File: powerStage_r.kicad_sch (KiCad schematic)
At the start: 19 parts, among them J3 motor

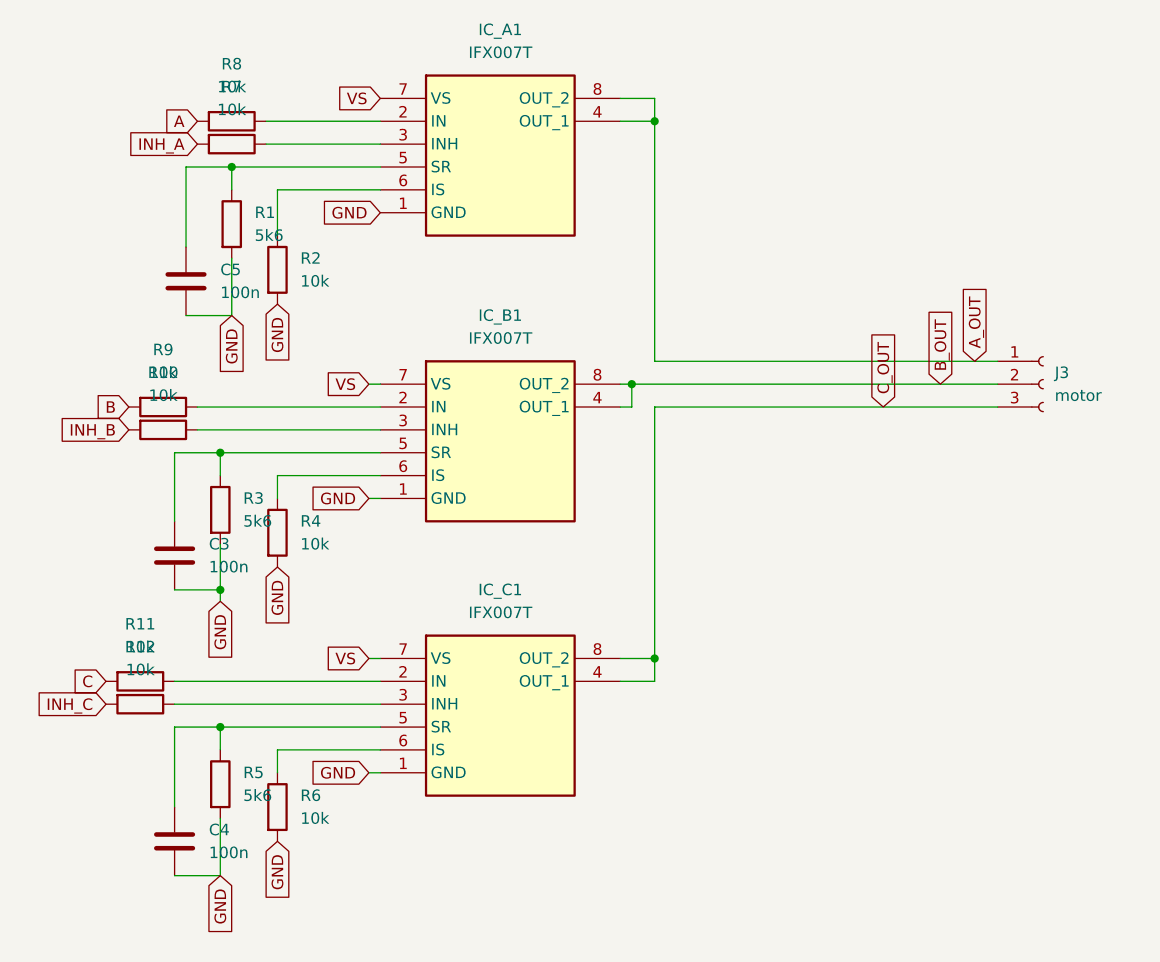
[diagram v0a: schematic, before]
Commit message: controller fw added, unfinished
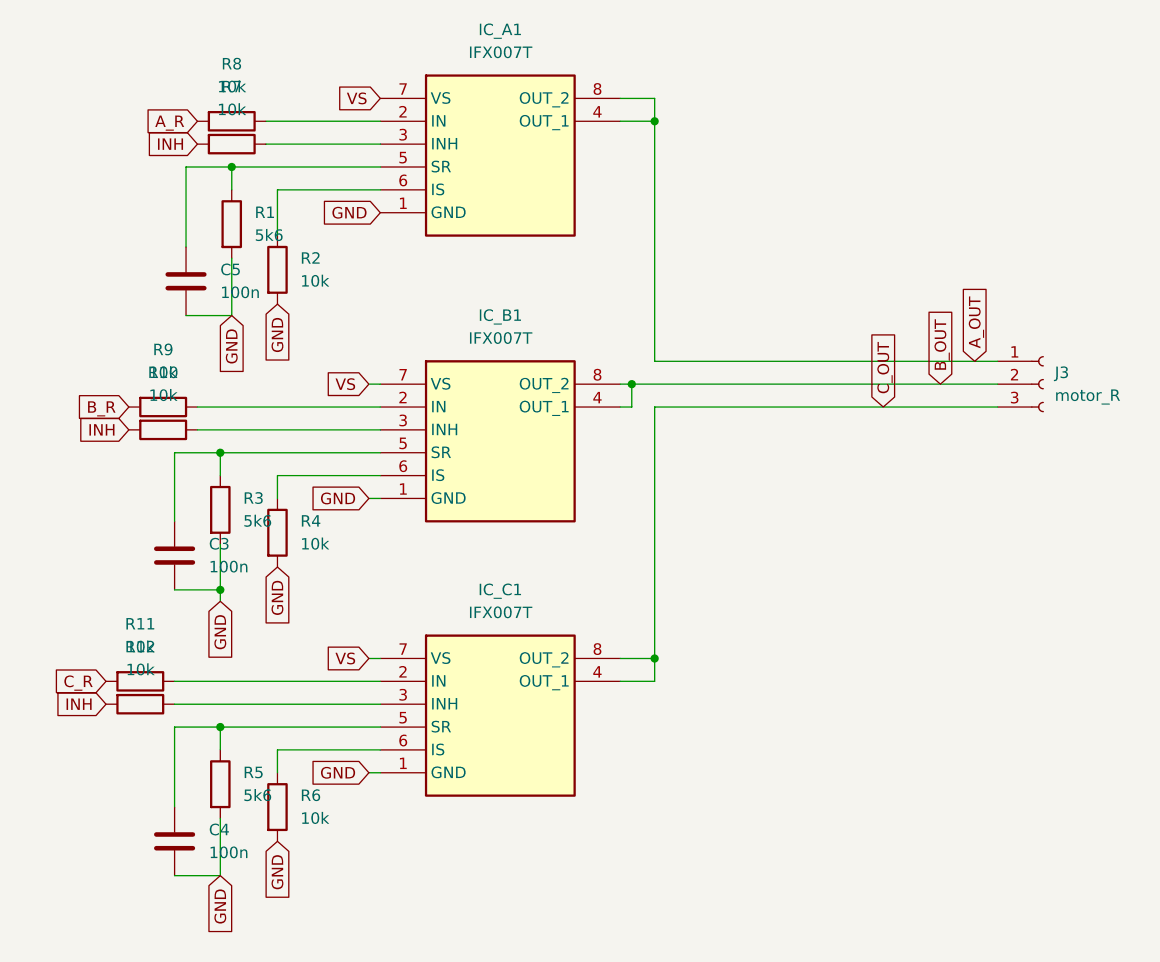
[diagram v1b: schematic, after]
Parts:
- J3: value motor -> motor_R
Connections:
- net INH_B is gone; now on net INH: R10.2
- net INH_C is gone; now on net INH: R12.2
- net A renamed A_R
- net B renamed B_R
- net C renamed C_R
- net INH_A renamed INH
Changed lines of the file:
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@@
 		)
 	)
-	(global_label "B"
+	(global_label "B_R"
 		(shape input)
 		(at 101.6 86.36 180)
@@
 		)
 		(property "Intersheetrefs" "${INTERSHEET_REFS}"
-			(at 97.3448 86.36 0)
+			(at 95.1072 86.36 0)
 			(effects
 				(font
@@
 		)
 	)
-	(global_label "INH_B"
+	(global_label "INH"
 		(shape input)
 		(at 101.6 88.9 180)
@@
 		)
 		(property "Intersheetrefs" "${INTERSHEET_REFS}"
-			(at 93.1114 88.9 0)
+			(at 95.349 88.9 0)
 			(effects
 				(font
@@
 		)
 	)
-	(global_label "A"
+	(global_label "A_R"
 		(shape input)
 		(at 109.22 54.61 180)
@@
 		)
 		(property "Intersheetrefs" "${INTERSHEET_REFS}"
-			(at 105.1462 54.61 0)
+			(at 102.9086 54.61 0)
 			(effects
 				(font
@@
 		)
 	)
-	(global_label "C"
+	(global_label "C_R"
 		(shape input)
 		(at 99.06 116.84 180)
@@
 		)
 		(property "Intersheetrefs" "${INTERSHEET_REFS}"
-			(at 94.8048 116.84 0)
+			(at 92.5672 116.84 0)
 			(effects
 				(font
@@
 		)
 	)
-	(global_label "INH_C"
+	(global_label "INH"
 		(shape input)
 		(at 99.06 119.38 180)
@@
 		)
 		(property "Intersheetrefs" "${INTERSHEET_REFS}"
-			(at 90.5714 119.38 0)
+			(at 92.809 119.38 0)
 			(effects
 				(font
@@
 		)
 	)
-	(global_label "INH_A"
+	(global_label "INH"
 		(shape input)
 		(at 109.22 57.15 180)
@@
 		)
 		(property "Intersheetrefs" "${INTERSHEET_REFS}"
-			(at 100.9128 57.15 0)
+			(at 102.969 57.15 0)
 			(effects
 				(font
@@
 			)
 		)
-		(property "Value" "motor"
+		(property "Value" "motor_R"
 			(at 204.47 85.09 0)
 			(effects
